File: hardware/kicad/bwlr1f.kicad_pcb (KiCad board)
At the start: 4 copper layers, 61.2 x 26.1 mm, 70 parts, among them J1 Conn_01x02, Q1 PMV32UP, Q2 PMV32UP, Q3 DMG1012UW, U1 RAK3172-SIP, U2 NBM7100ABQX, U3 ZD24C08A, U4 BME688, U5 TPL5110

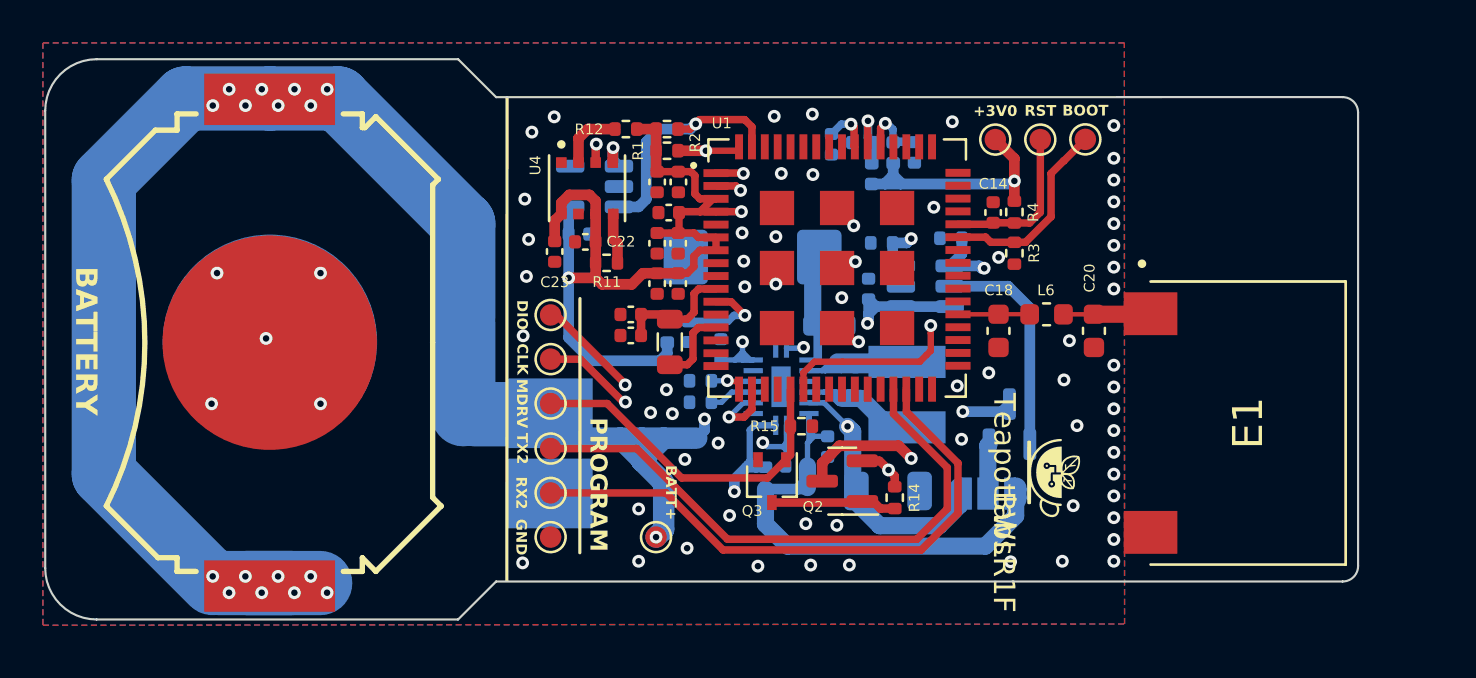
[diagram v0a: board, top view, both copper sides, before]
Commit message: change antenna
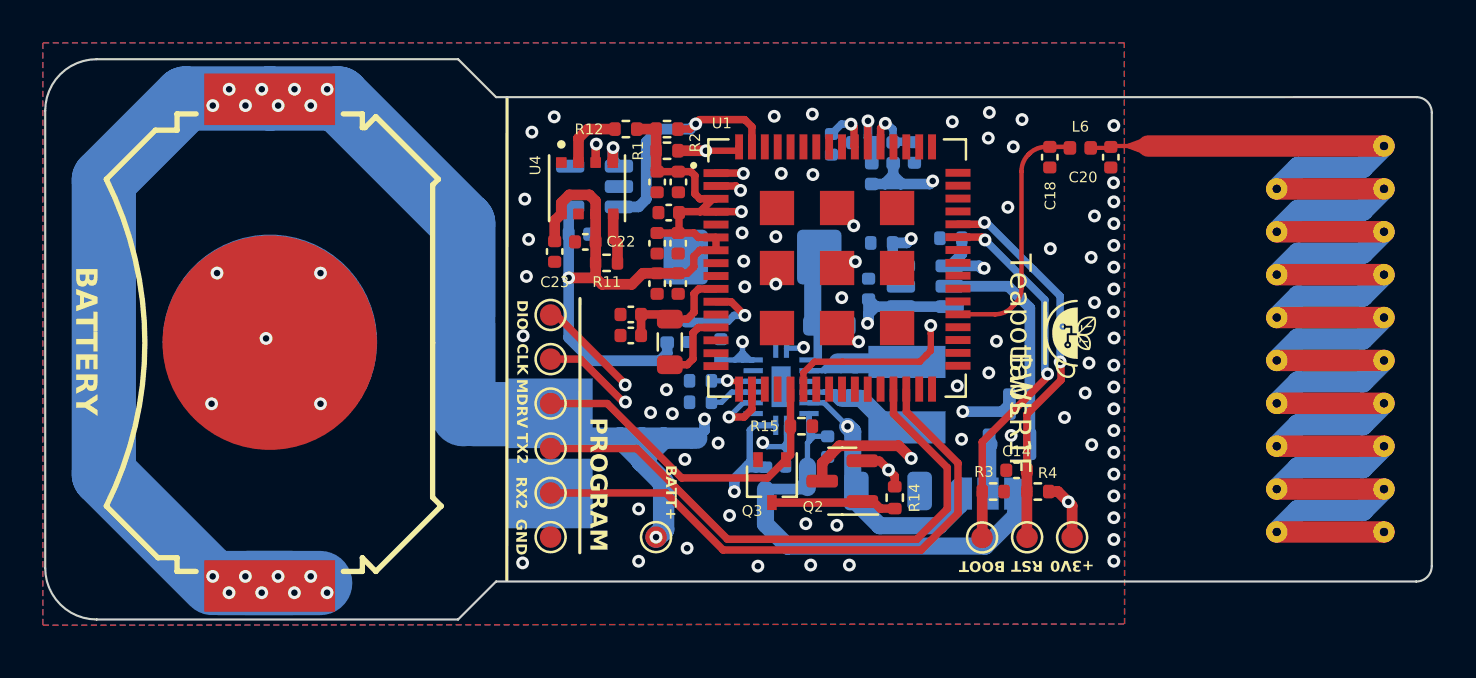
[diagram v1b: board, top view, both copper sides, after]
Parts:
- removed E1: ANT-915-USP410, bwlr1f:XDCR_ANT-915-USP410
- added AE1: Antenna, RF_Antenna:Texas_SWRA416_868MHz_915MHz, F.Cu at (162.1, 110.5)
- C18, C20: footprint Capacitor_SMD:C_0603_1608Metric -> Capacitor_SMD:C_0402_1005Metric
- L6: footprint Inductor_SMD:L_0603_1608Metric -> Inductor_SMD:L_0402_1005Metric
- moved TP6 19.2 mm to (149.2, 119.8), turned to -90 degrees
- moved TP8 18.9 mm to (153.4, 119.8), turned to 0 degrees
- moved TP5 18.6 mm to (151.3, 119.8), turned to -90 degrees
- moved R4 13.1 mm to (151.8, 117.7), turned to 180 degrees
- moved C14 12.1 mm to (150.8, 116.7), turned to 0 degrees
- moved R3 11.2 mm to (149.7, 117.7), turned to 0 degrees
- moved C18 8.45 mm to (152.3, 102.1)
- moved C20 8.14 mm to (155.2, 102.1)
- moved L6 7.92 mm to (153.7, 101.6)
- moved G*** 6.53 mm to (153.3, 110.5)
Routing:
- net /RST: track 7.47 -> 18.2 mm, vias 0 -> 2
- net /RF: track 3.34 -> 12.0 mm
- net /BOOT: track 9.21 -> 17.7 mm, vias 0 -> 2
- net +3V0: track 89.7 -> 93.8 mm, vias 5 -> 6
- net /ANT: track 4.07 -> 1.97 mm
- net GND: vias 69 -> 77
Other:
- board size 61.2 x 26.1 mm -> 64.7 x 26.1 mm
- board text added: "REVISION 2"
- board text removed: "REVISION 1"

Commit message: Revert "change antenna"
This reverts commit 46c20b2a2dd1e0a5efdce99ceacd3ab7d772dc0d.
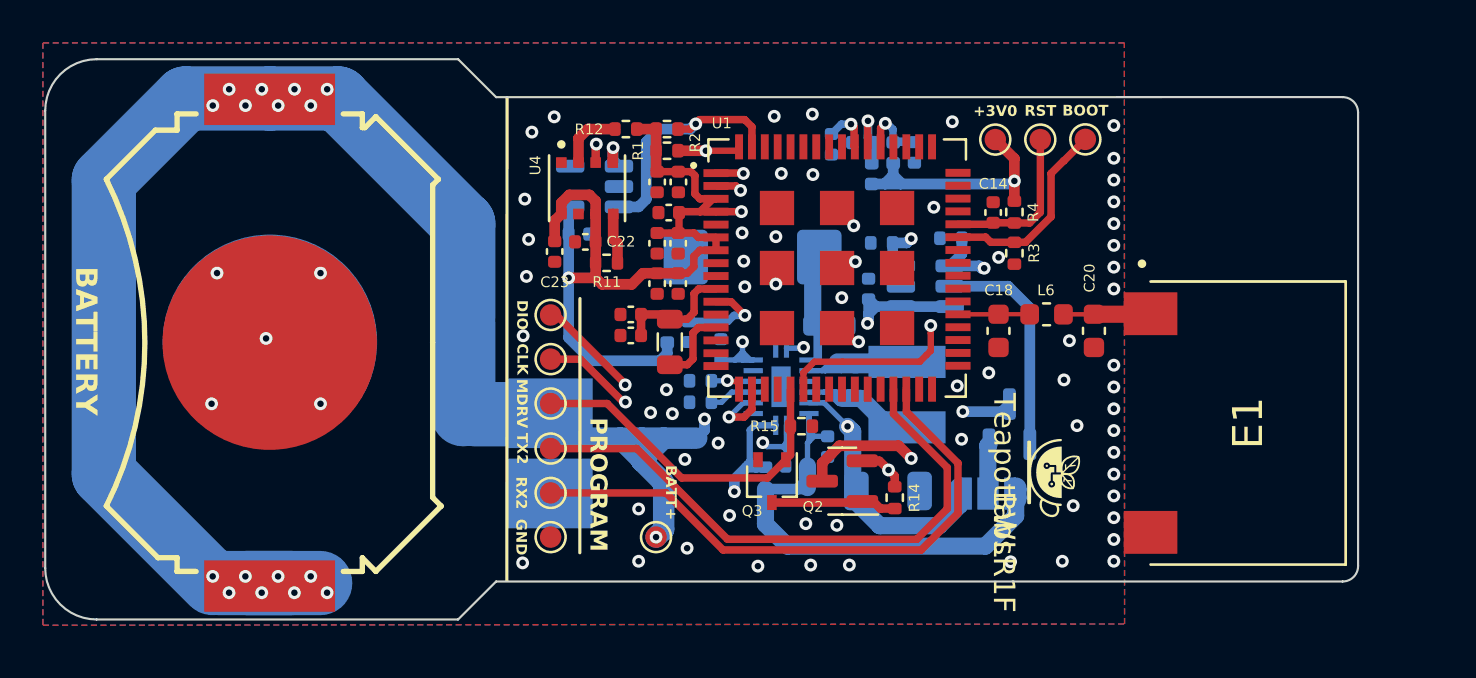
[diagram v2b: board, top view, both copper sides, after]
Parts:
- removed AE1: Antenna, RF_Antenna:Texas_SWRA416_868MHz_915MHz
- added E1: ANT-915-USP410, bwlr1f:XDCR_ANT-915-USP410, F.Cu at (161.6, 114.5)
- C18, C20: footprint Capacitor_SMD:C_0402_1005Metric -> Capacitor_SMD:C_0603_1608Metric
- L6: footprint Inductor_SMD:L_0402_1005Metric -> Inductor_SMD:L_0603_1608Metric
- moved TP6 19.2 mm to (154.0, 101.2), turned to 90 degrees
- moved TP8 18.9 mm to (149.8, 101.2), turned to 180 degrees
- moved TP5 18.6 mm to (151.9, 101.2), turned to 90 degrees
- moved R4 13.1 mm to (150.7, 104.6), turned to -90 degrees
- moved C14 12.1 mm to (149.7, 104.6), turned to -90 degrees
- moved R3 11.2 mm to (150.7, 106.5), turned to -90 degrees
- moved C18 8.45 mm to (149.9, 110.2)
- moved C20 8.14 mm to (154.4, 110.2)
- moved L6 7.92 mm to (152.2, 109.4)
- moved G*** 6.53 mm to (152.5, 117.0)
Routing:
- net /RST: track 18.2 -> 7.47 mm, vias 2 -> 0
- net /RF: track 12.0 -> 3.34 mm
- net /BOOT: track 17.7 -> 9.21 mm, vias 2 -> 0
- net +3V0: track 93.8 -> 89.7 mm, vias 6 -> 5
- net /ANT: track 1.97 -> 4.07 mm
- net GND: vias 77 -> 69
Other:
- board size 64.7 x 26.1 mm -> 61.2 x 26.1 mm
- board text added: "REVISION 1"
- board text removed: "REVISION 2"
